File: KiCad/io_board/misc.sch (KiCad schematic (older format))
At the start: 10 parts, among them U6 27C512

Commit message: Working on IO board
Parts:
- C10, C11: footprint Capacitor_THT:C_Disc_D4.3mm_W1.9mm_P5.00mm -> Capacitor_SMD:C_1206_3216Metric
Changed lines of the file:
@@
 $Descr A4 11693 8268
 encoding utf-8
-Sheet 7 7
+Sheet 7 8
 Title "Mini8086 I/O board"
 Date "2020-11-05"
@@
 F 0 "C10" H 7015 3546 50  0000 L CNN
 F 1 "100n" H 7015 3455 50  0000 L CNN
-F 2 "Capacitor_THT:C_Disc_D4.3mm_W1.9mm_P5.00mm" H 6938 3350 50  0001 C CNN
+F 2 "Capacitor_SMD:C_1206_3216Metric" H 6938 3350 50  0001 C CNN
 F 3 "~" H 6900 3500 50  0001 C CNN
 	1    6900 3500
@@
 F 0 "C11" H 7465 3546 50  0000 L CNN
 F 1 "100n" H 7465 3455 50  0000 L CNN
-F 2 "Capacitor_THT:C_Disc_D4.3mm_W1.9mm_P5.00mm" H 7388 3350 50  0001 C CNN
+F 2 "Capacitor_SMD:C_1206_3216Metric" H 7388 3350 50  0001 C CNN
 F 3 "~" H 7350 3500 50  0001 C CNN
 	1    7350 3500

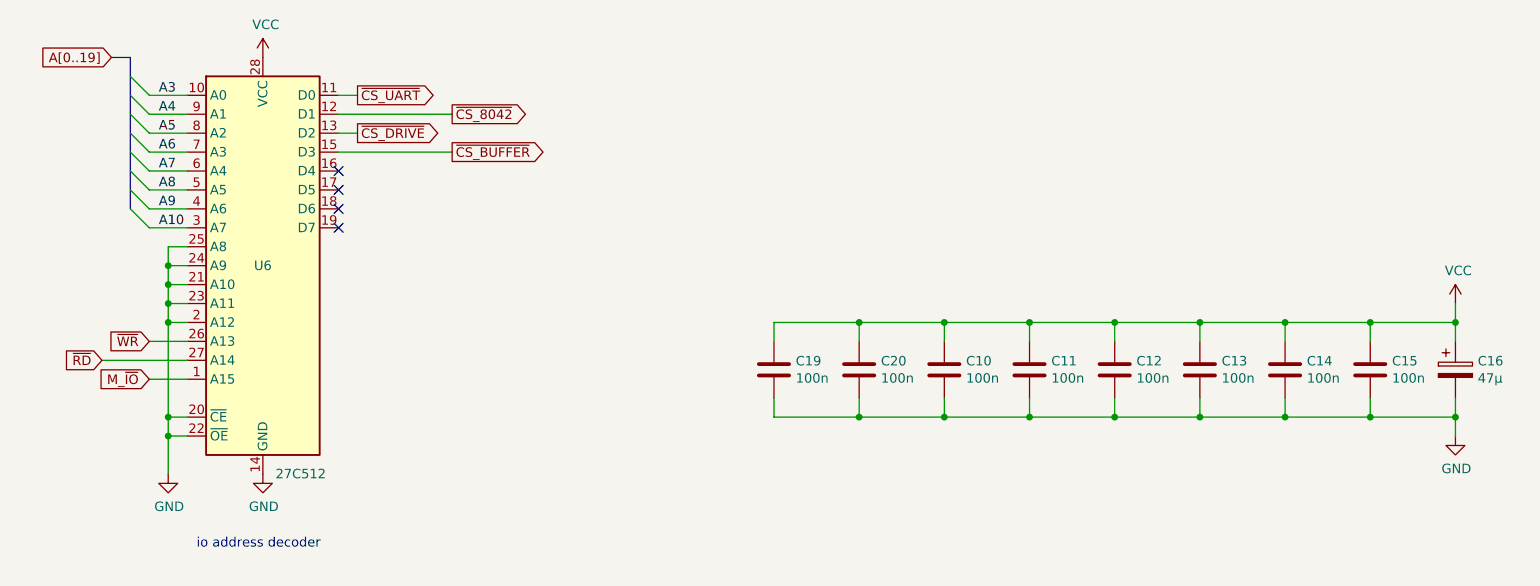
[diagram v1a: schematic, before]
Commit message: Worked on I/O board.
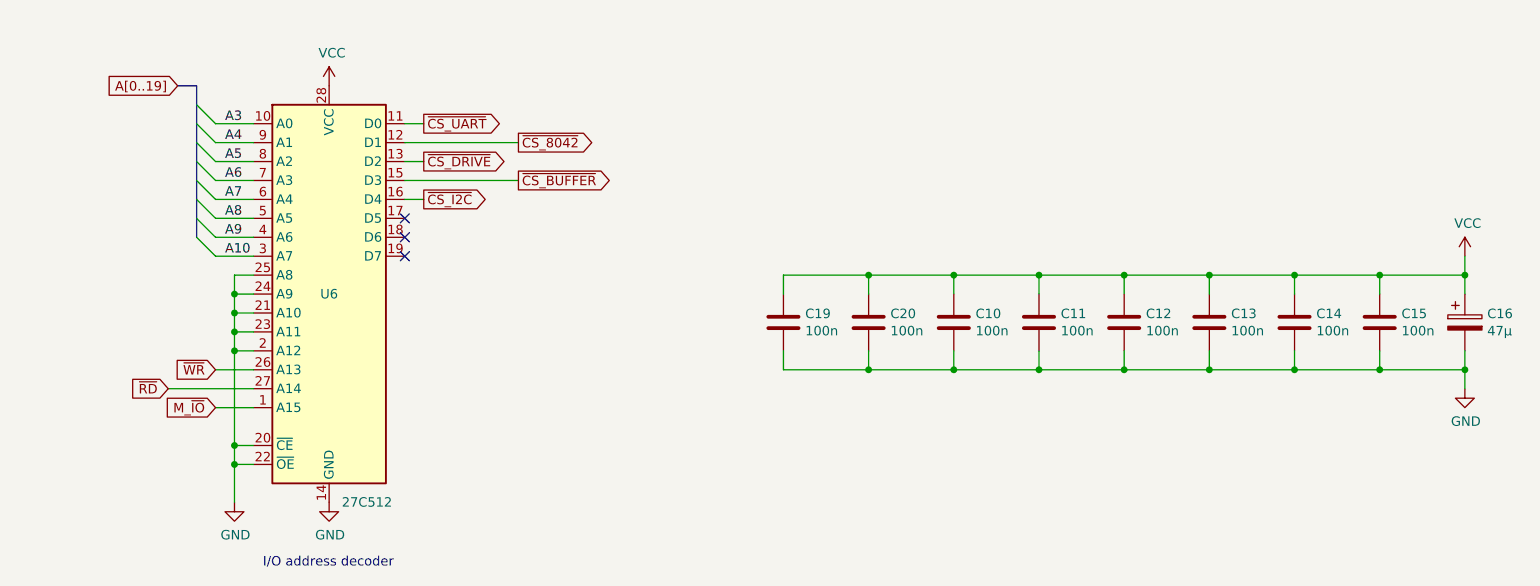
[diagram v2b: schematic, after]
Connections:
- net ~CS_I2C: now reaches U6.16 (D4)
- no-connect marks 4 -> 3
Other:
- note added: "I/O address decoder"
- note removed: "io address decoder"
- moved on the sheet: C10, C11, C12, C13, C14, C15, C16, C19, C20, U6
